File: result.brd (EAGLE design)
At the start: 900 x 880 mm, 0 parts

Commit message: !U heated bed calculator
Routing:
- net SIGNAL1: track 57461.0 -> 6291.0 mm
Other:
- board size 900 x 880 mm -> 110 x 110 mm

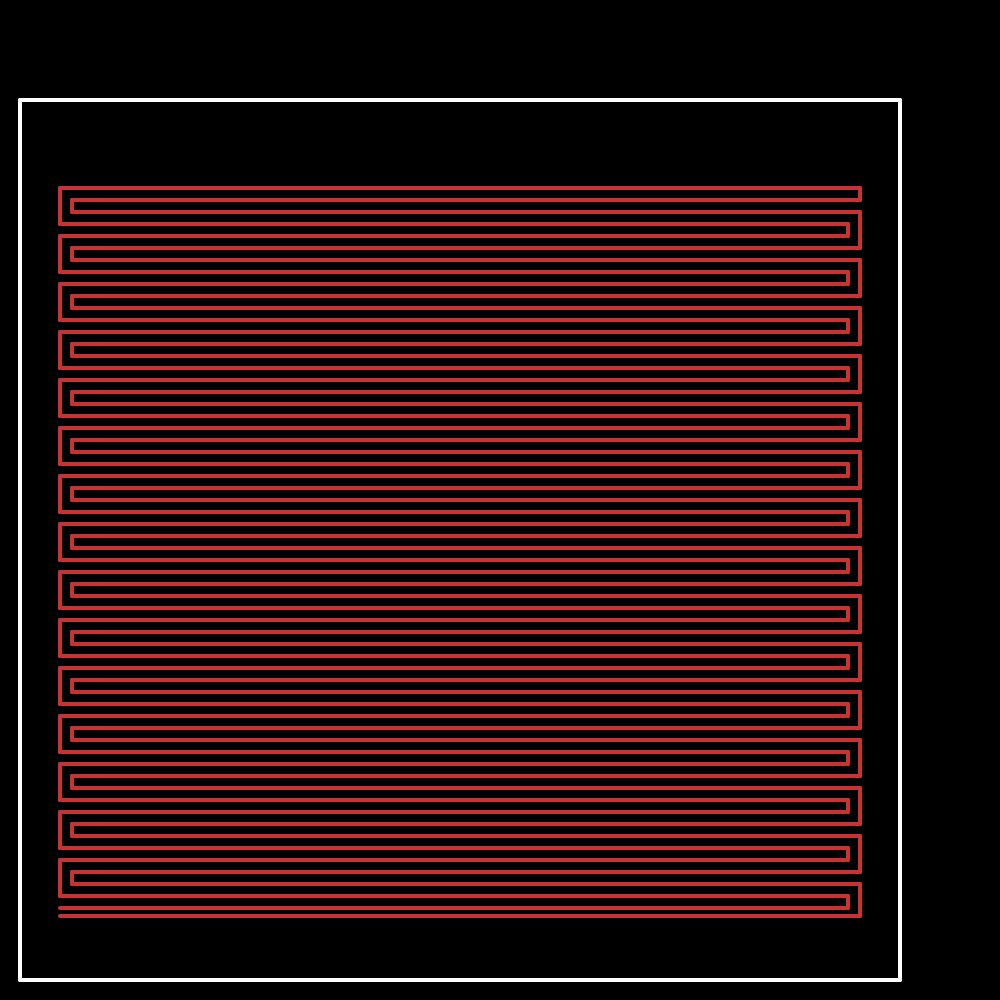
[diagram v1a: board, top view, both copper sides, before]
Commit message: !U processing 3
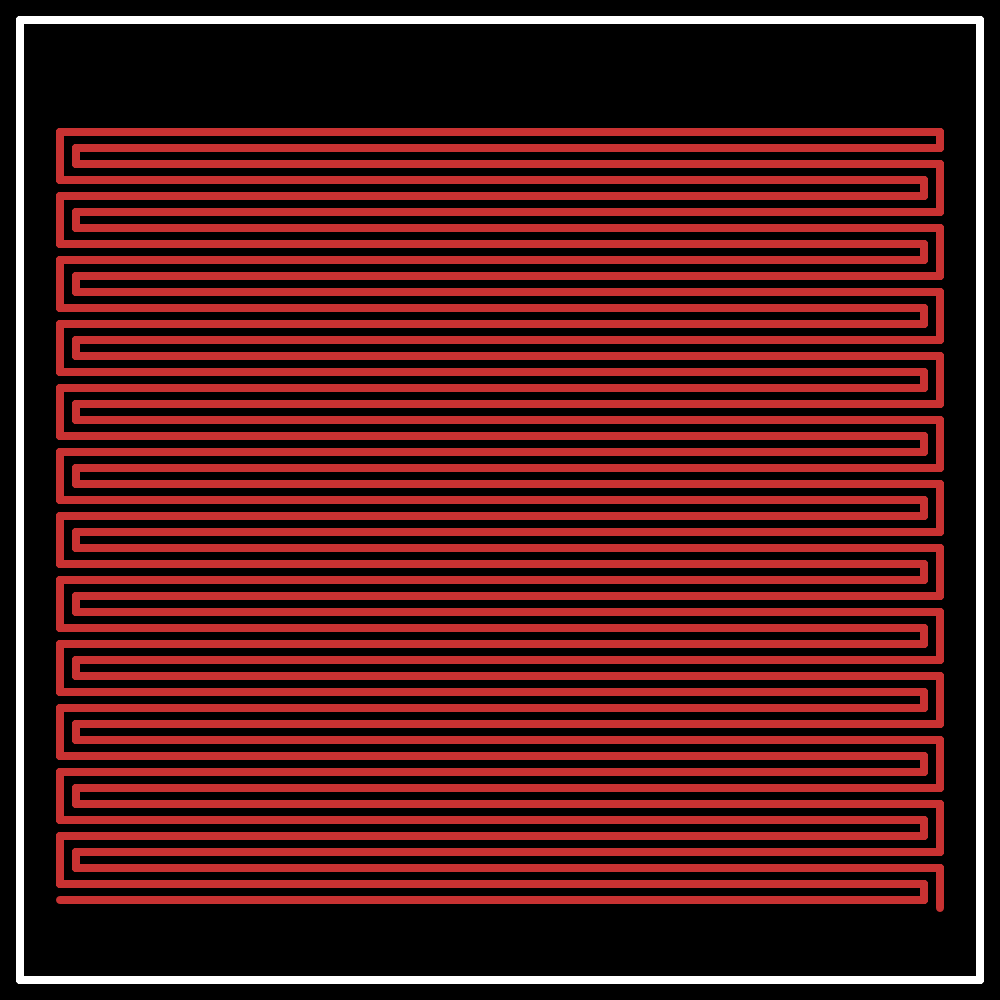
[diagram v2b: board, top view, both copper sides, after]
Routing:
- net SIGNAL1: track 6291.0 -> 5487.0 mm
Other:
- board size 110 x 110 mm -> 120 x 120 mm
